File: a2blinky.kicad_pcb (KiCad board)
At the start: 2 copper layers, 75 x 75 mm, 26 parts, among them J1 Barrel_Jack_Switch, U1 74HC164, U2 4002, U3 AP1117-33, U4 LMC555xM

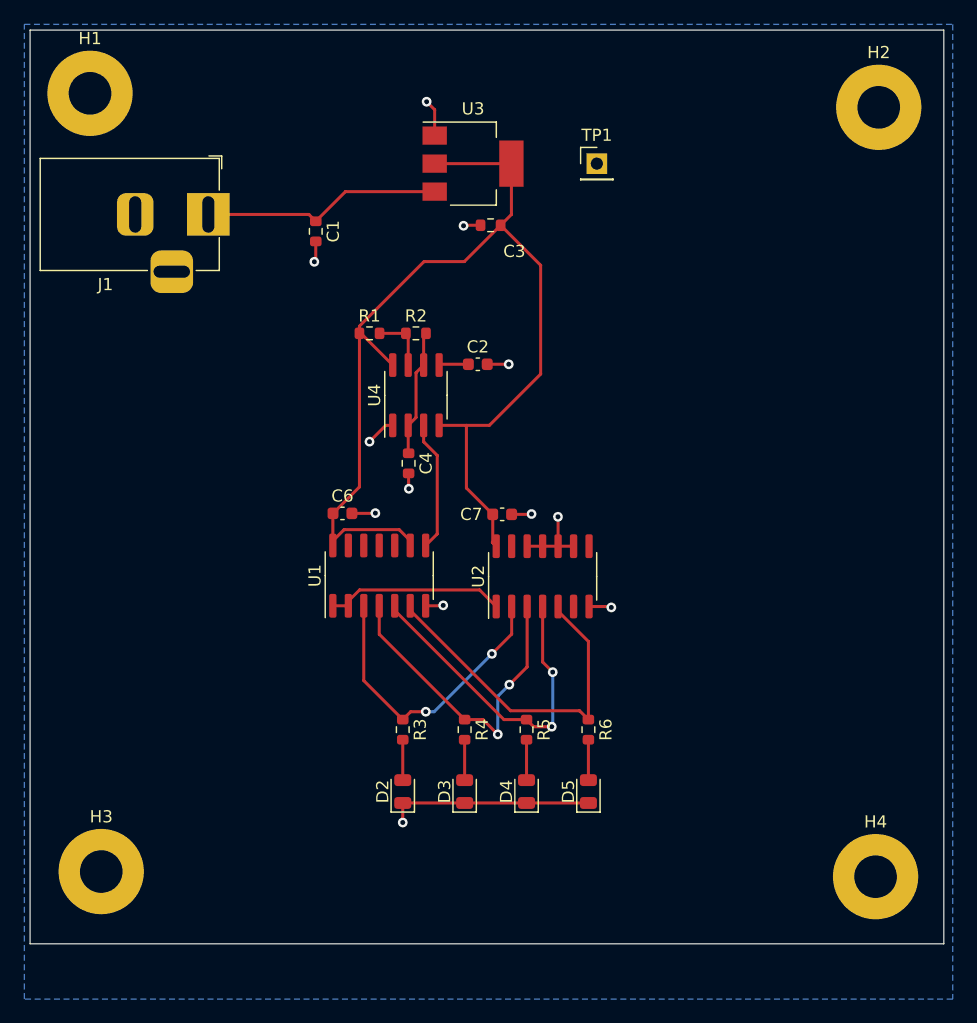
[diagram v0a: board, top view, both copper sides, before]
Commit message: ecos
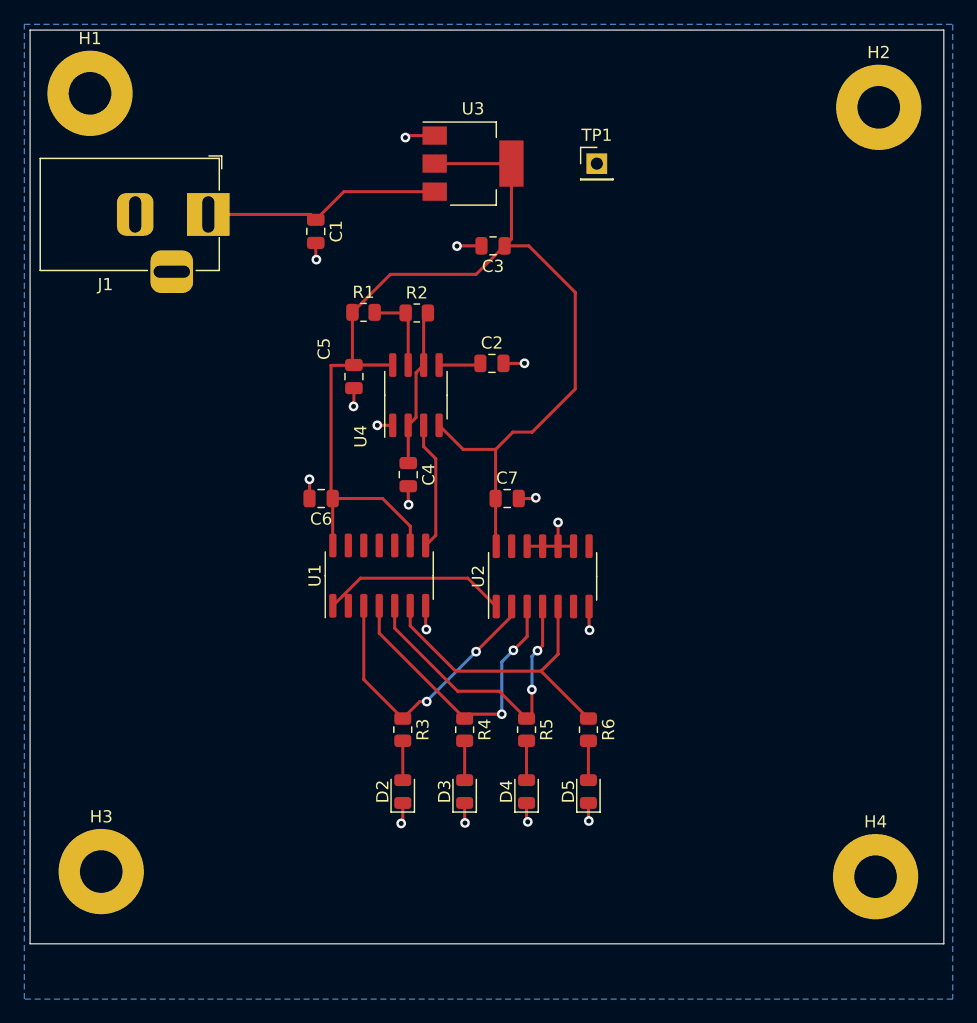
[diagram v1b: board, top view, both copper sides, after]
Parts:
- added C5: 100n, Capacitor_SMD:C_0805_2012Metric, F.Cu at (76.6, 78.4)
- C1, C3, C4: footprint Resistor_SMD:R_0603_1608Metric -> Capacitor_SMD:C_0805_2012Metric
- C2, C6, C7: footprint Capacitor_SMD:C_0603_1608Metric -> Capacitor_SMD:C_0805_2012Metric
- R1, R2, R3, R4, R5, R6: footprint Resistor_SMD:R_0603_1608Metric -> Resistor_SMD:R_0805_2012Metric
- moved C6 2.13 mm to (73.9, 88.5), turned to 180 degrees
- moved R1 1.79 mm to (77.4, 73.2)
- moved C3 1.70 mm to (88.0, 67.7)
- moved R2 1.67 mm to (81.7, 73.2)
- moved C7 1.36 mm to (89.2, 88.5)
- moved C2 1.16 mm to (87.9, 77.4)
- moved C4 0.93 mm to (81.0, 86.5)
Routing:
- net GND: track 41.7 -> 31.1 mm, vias 12 -> 16
- net VCC: track 92.4 -> 98.6 mm
- net Net-(R6-Pad1): track 29.0 -> 25.3 mm
- net Net-(C4-Pad1): track 10.5 -> 13.0 mm
- net Net-(R1-Pad2): track 4.84 -> 6.93 mm
- net Net-(R5-Pad1): track 27.5 -> 25.5 mm
- net Net-(R4-Pad1): track 27.0 -> 25.1 mm
- net Net-(C2-Pad1): track 2.43 -> 3.44 mm
- net Net-(R3-Pad1): track 24.8 -> 23.8 mm
- net Net-(U1-Pad1): track 14.7 -> 15.3 mm
